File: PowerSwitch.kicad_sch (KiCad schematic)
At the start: 16 parts, among them U401 BTT6010

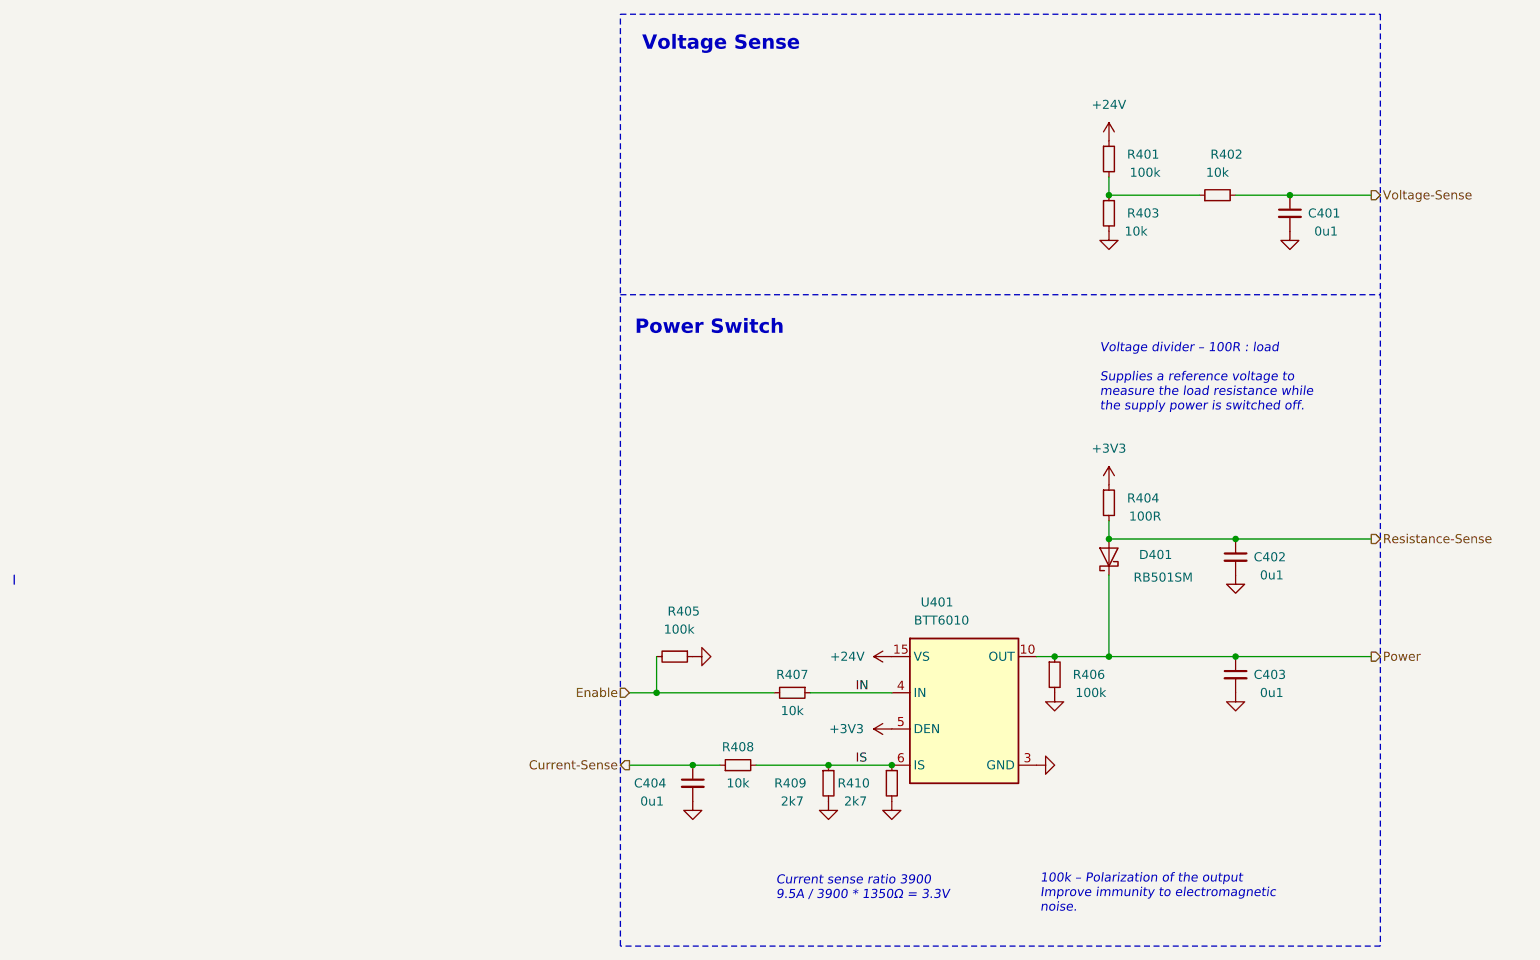
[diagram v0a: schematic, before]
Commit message: Update parts
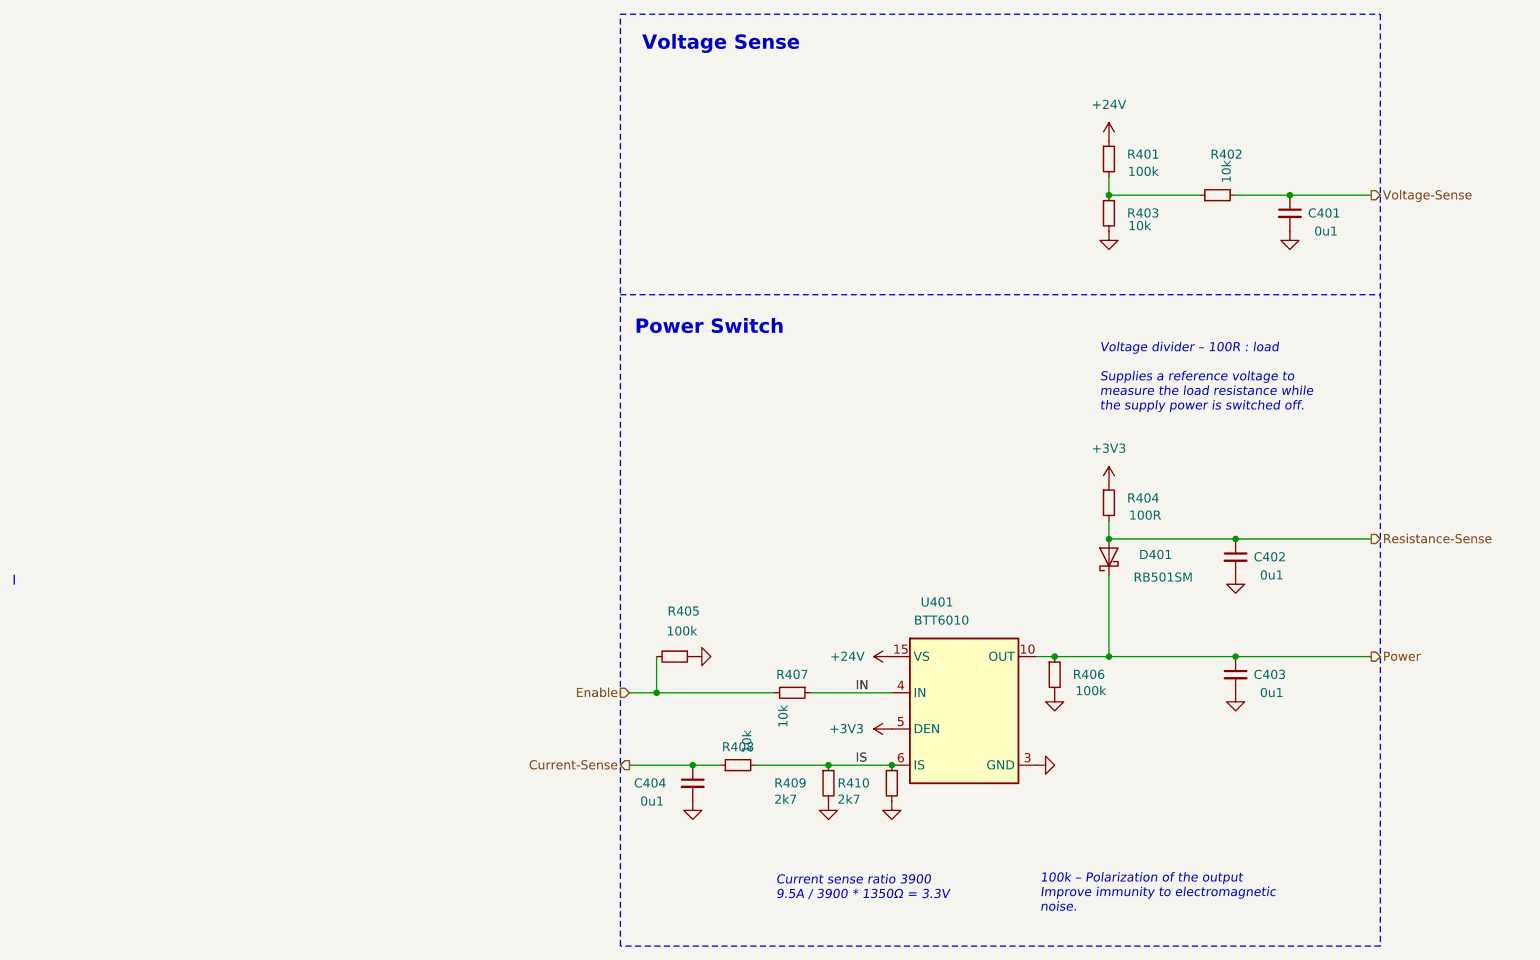
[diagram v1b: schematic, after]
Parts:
- C401, C402, C403, C404: footprint Capacitor_SMD:C_0603_1608Metric -> V2_Capacitor_SMD:C_0603; symbol Device:C_Small -> V2_Device:C_0603_0u1; Manufacturer (none) -> TDK; Mouser (none) -> 810-CGA3E2X7R1H104MA; Product (none) -> CGA3E2X7R1H104M080AA
- D401: footprint Diode_SMD:D_SOD-523 -> V2_Diode_SMD:D_SOD-523; Manufacaturer (none) -> ROHM Semiconductor; Manufacturer (none) -> ROHM Semiconductor; Mouser (none) -> 755-RB501SM-30FHT2R; Product (none) -> RB501SM-30FHT2R
- R401, R405, R406: footprint Resistor_SMD:R_0603_1608Metric -> V2_Resistor_SMD:R_0603; symbol Device:R_Small -> V2_Device:R_0603_100k; Manufacturer (none) -> Vishay; Mouser (none) -> 71-CRCW0603100KFKEAC; Product (none) -> CRCW0603100KFKEAC; Rating (none) -> 100mW
- R402, R403, R407, R408: footprint Resistor_SMD:R_0603_1608Metric -> V2_Resistor_SMD:R_0603; symbol Device:R_Small -> V2_Device:R_0603_10k; Manufacturer (none) -> Vishay; Mouser (none) -> 71-CRCW060310K0FKEAC; Product (none) -> CRCW060310K0FKEAC; Rating (none) -> 100mW
- R404: footprint Resistor_SMD:R_0603_1608Metric -> V2_Resistor_SMD:R_0603; symbol Device:R_Small -> V2_Device:R_0603_100R; Manufacturer (none) -> Vishay; Mouser (none) -> 71-CRCW0603100RFKEAH; Product (none) -> CRCW0603100RFKEAHP; Rating (none) -> 330mW
- R409, R410: footprint Resistor_SMD:R_0603_1608Metric -> V2_Resistor_SMD:R_0603; symbol Device:R_Small -> V2_Device:R_0603_2k7; Manufacturer (none) -> Vishay; Mouser (none) -> 71-CRCW06032K70FKEAC; Product (none) -> CRCW06032K70FKEAC; Rating (none) -> 100mW
- U401: Manufacturer (none) -> Infineon; Mouser (none) -> 726-BTT60101ERBXUMA1; Product (none) -> BTT60101ERBXUMA1
